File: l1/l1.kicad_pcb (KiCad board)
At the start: 2 copper layers, 122 x 122 mm, 60 parts

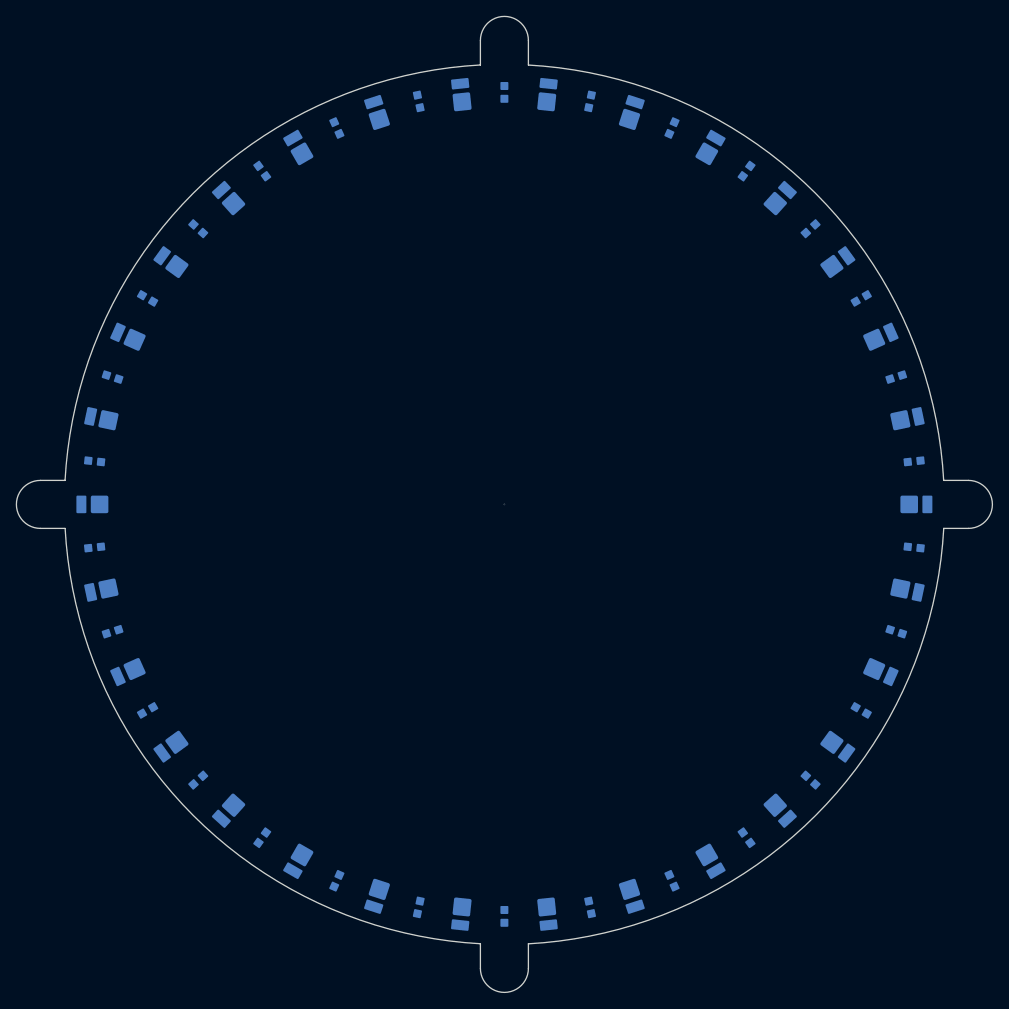
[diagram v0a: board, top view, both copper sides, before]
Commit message: 死
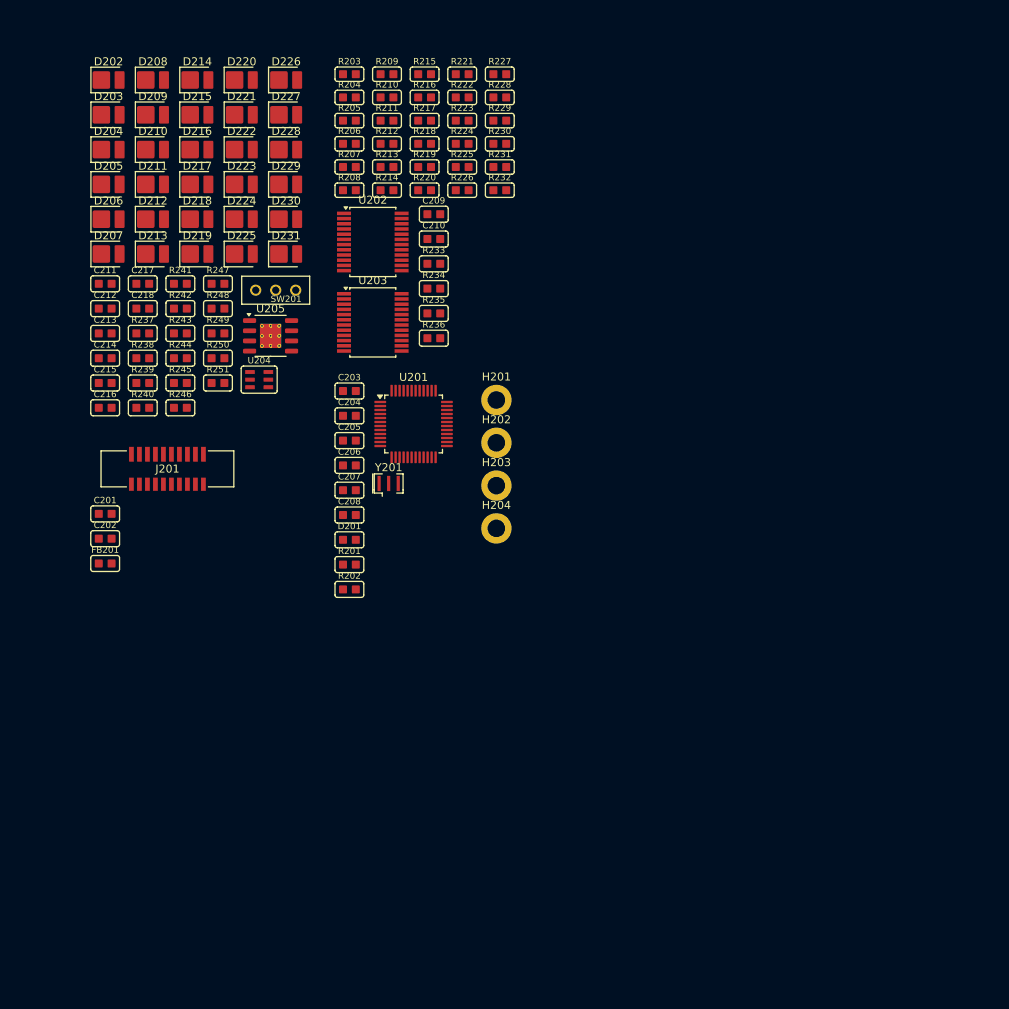
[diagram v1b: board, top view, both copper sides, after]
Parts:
- removed R252, R253, R254, R255, R256, R257, R258, R259, R260, R261, R262, R263, R264: R, Library:res0603
- added C201: 2u2, Library:cap0603, F.Cu at (105.3, 111.2)
- added C202: 2u2, Library:cap0603, F.Cu at (105.3, 114.3)
- added C203: 2u2, Library:cap0603, F.Cu at (135.8, 95.8)
- added C204: 0u1, Library:cap0603, F.Cu at (135.8, 98.9)
- added C205: 0u1, Library:cap0603, F.Cu at (135.8, 102.0)
- added C206: 0u1, Library:cap0603, F.Cu at (135.8, 105.1)
- added C207: 0u1, Library:cap0603, F.Cu at (135.8, 108.2)
- added C208: 0u1, Library:cap0603, F.Cu at (135.8, 111.3)
- added C209: 0u1, Library:cap0603, F.Cu at (146.4, 73.7)
- added C210: 0u1, Library:cap0603, F.Cu at (146.4, 76.8)
- added C211: 0u1, Library:cap0603, F.Cu at (105.3, 82.4)
- added C212: 10n, Library:cap0603, F.Cu at (105.3, 85.5)
- added C213: 10u, Library:cap0603, F.Cu at (105.3, 88.6)
- added C214: 22u, Library:cap0603, F.Cu at (105.3, 91.7)
- added C215: 0u1, Library:cap0603, F.Cu at (105.3, 94.8)
- added C216: 22u, Library:cap0603, F.Cu at (105.3, 97.9)
- added C217: 1u, Library:cap0603, F.Cu at (110.0, 82.4)
- added C218: 0u1, Library:cap0603, F.Cu at (110.0, 85.5)
- added D231: LED, Library:led2835, F.Cu at (127.9, 78.7)
- added FB201: 100R, Library:fb0603, F.Cu at (105.3, 117.4)
- added H201: MountingHole, MountingHole:MountingHole_2.2mm_M2_ISO14580_Pad, F.Cu at (154.2, 97.0)
- added H202: MountingHole, MountingHole:MountingHole_2.2mm_M2_ISO14580_Pad, F.Cu at (154.2, 102.3)
- added H203: MountingHole, MountingHole:MountingHole_2.2mm_M2_ISO14580_Pad, F.Cu at (154.2, 107.7)
- added H204: MountingHole, MountingHole:MountingHole_2.2mm_M2_ISO14580_Pad, F.Cu at (154.2, 113.0)
- added J201: Conn_01x10, Library:526101071, F.Cu at (113.1, 105.6)
- added R201: R, Library:res0603, F.Cu at (135.8, 117.5)
- added R202: 1K, Library:res0603, F.Cu at (135.8, 120.6)
- added R203: R_Photo, Library:als-pt19, F.Cu at (135.8, 56.2)
- added R204: R_Photo, Library:als-pt19, F.Cu at (135.8, 59.1)
- added R205: R_Photo, Library:als-pt19, F.Cu at (135.8, 62.0)
- added R206: R_Photo, Library:als-pt19, F.Cu at (135.8, 64.9)
- added R207: R_Photo, Library:als-pt19, F.Cu at (135.8, 67.8)
- added R208: R_Photo, Library:als-pt19, F.Cu at (135.8, 70.7)
- added R209: R_Photo, Library:als-pt19, F.Cu at (140.5, 56.2)
- added R210: R_Photo, Library:als-pt19, F.Cu at (140.5, 59.1)
- added R211: R_Photo, Library:als-pt19, F.Cu at (140.5, 62.0)
- added R212: R_Photo, Library:als-pt19, F.Cu at (140.5, 64.9)
- added R213: R_Photo, Library:als-pt19, F.Cu at (140.5, 67.8)
- added R214: R_Photo, Library:als-pt19, F.Cu at (140.5, 70.7)
- added R215: R_Photo, Library:als-pt19, F.Cu at (145.2, 56.2)
- added R216: R_Photo, Library:als-pt19, F.Cu at (145.2, 59.1)
- added R217: R_Photo, Library:als-pt19, F.Cu at (145.2, 62.0)
- added R218: R_Photo, Library:als-pt19, F.Cu at (145.2, 64.9)
- added R219: R_Photo, Library:als-pt19, F.Cu at (145.2, 67.8)
- added R220: R_Photo, Library:als-pt19, F.Cu at (145.2, 70.7)
- added R221: R_Photo, Library:als-pt19, F.Cu at (149.9, 56.2)
- added R222: R_Photo, Library:als-pt19, F.Cu at (149.9, 59.1)
- added R223: R_Photo, Library:als-pt19, F.Cu at (149.9, 62.0)
- added R224: R_Photo, Library:als-pt19, F.Cu at (149.9, 64.9)
- added R225: R_Photo, Library:als-pt19, F.Cu at (149.9, 67.8)
- added R226: R_Photo, Library:als-pt19, F.Cu at (149.9, 70.7)
- added R227: R_Photo, Library:als-pt19, F.Cu at (154.6, 56.2)
- added R228: R_Photo, Library:als-pt19, F.Cu at (154.6, 59.1)
- added R229: R_Photo, Library:als-pt19, F.Cu at (154.6, 62.0)
- added R230: R_Photo, Library:als-pt19, F.Cu at (154.6, 64.9)
- added R231: R_Photo, Library:als-pt19, F.Cu at (154.6, 67.8)
- added R232: R_Photo, Library:als-pt19, F.Cu at (154.6, 70.7)
- added R233: 3K24, Library:res0603, F.Cu at (146.4, 79.9)
- added R234: 10K, Library:res0603, F.Cu at (146.4, 83.0)
- added SW201: SW_SPDT, Library:SS12D00G3, F.Cu at (126.6, 83.2)
- added U201: STM32F103CBTX, Package_QFP:LQFP-48_7x7mm_P0.5mm, F.Cu at (143.8, 100.0)
- added U202: CD74HC4067SM, Package_SO:SSOP-24_5.3x8.2mm_P0.65mm, F.Cu at (138.8, 77.2)
- added U203: CD74HC4067SM, Package_SO:SSOP-24_5.3x8.2mm_P0.65mm, F.Cu at (138.8, 87.2)
- added U204: TPS22917x, Library:SOT-23-6, F.Cu at (124.5, 94.4)
- added U205: ILD8150, Package_SO:Infineon_PG-DSO-8-27_3.9x4.9mm_EP2.65x3mm_ThermalVias, F.Cu at (126.0, 88.9)
- added Y201: 8Mhz, Crystal:Resonator_SMD_Murata_CSTxExxV-3Pin_3.0x1.1mm, F.Cu at (140.7, 107.4)
- D201: value LED -> RED; footprint Library:led2835 -> Library:led0603; moved to F.Cu
- D202, D203, D204, D205, D206, D207, D208, D209, D210, D211, D212, D213, D214, D215, D216, D217, D218, D219, D220, D221, D222, D223, D224, D225, D226, D227, D228, D229, D230, R250: moved to F.Cu
- R235: value R -> 3K24; moved to F.Cu
- R236, R249: value R -> 10K; moved to F.Cu
- R237, R238, R239, R240, R241, R242, R243, R244, R245, R246: value R -> 150; moved to F.Cu
- R247: value R -> 100K; moved to F.Cu
- R248: value R -> 1; moved to F.Cu
- R251: value R -> 0.3; moved to F.Cu
- moved D214 113.0 mm to (116.8, 57.0), turned to 0 degrees
- moved D209 111.4 mm to (111.3, 61.3), turned to 0 degrees
- moved D208 111.2 mm to (111.3, 57.0), turned to 0 degrees
- moved D210 110.9 mm to (111.3, 65.7), turned to 0 degrees
- moved D211 109.6 mm to (111.3, 70.0), turned to 0 degrees
- moved D212 107.7 mm to (111.3, 74.3), turned to 0 degrees
- moved D215 106.8 mm to (116.8, 61.3), turned to 0 degrees
- moved D213 105.4 mm to (111.3, 78.7), turned to 0 degrees
- moved D216 100.2 mm to (116.8, 65.7)
- moved R241 99.5 mm to (114.7, 82.4), turned to 0 degrees
- moved R240 97.4 mm to (110.0, 97.9), turned to 0 degrees
- moved R239 97.1 mm to (110.0, 94.8), turned to 0 degrees
- moved R242 96.5 mm to (114.7, 85.5), turned to 0 degrees
- moved R238 96.4 mm to (110.0, 91.7), turned to 0 degrees
- moved R237 95.2 mm to (110.0, 88.6), turned to 0 degrees
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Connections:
- D201 pad 2: +3V3 -> /Light Ring/STM32/MCU1 LED
- D202 pad 1: Net-(D201-K) -> Net-(D202-K)
- D202 pad 2: +3V3 -> /Light Ring/LED/LED VIN
- D203 pad 1: Net-(D201-K) -> Net-(D203-K)
- D203 pad 2: +3V3 -> /Light Ring/LED/LED VIN
- D204 pad 1: Net-(D201-K) -> Net-(D204-K)
- D204 pad 2: +3V3 -> /Light Ring/LED/LED VIN
- D205 pad 1: Net-(D201-K) -> Net-(D205-K)
- D205 pad 2: +3V3 -> /Light Ring/LED/LED VIN
- D206 pad 1: Net-(D201-K) -> Net-(D206-K)
- D206 pad 2: +3V3 -> /Light Ring/LED/LED VIN
- D207 pad 1: Net-(D201-K) -> Net-(D207-K)
- D207 pad 2: +3V3 -> /Light Ring/LED/LED VIN
- D208 pad 1: Net-(D201-K) -> Net-(D208-K)
- D208 pad 2: +3V3 -> /Light Ring/LED/LED VIN
- D209 pad 1: Net-(D201-K) -> Net-(D209-K)
- D209 pad 2: +3V3 -> /Light Ring/LED/LED VIN
- D210 pad 1: Net-(D201-K) -> Net-(D210-K)
- D210 pad 2: +3V3 -> /Light Ring/LED/LED VIN
- D211 pad 1: Net-(D201-K) -> Net-(D211-K)
- D211 pad 2: +3V3 -> /Light Ring/LED/LED VIN
- D212 pad 1: Net-(D201-K) -> Net-(D212-K)
- D212 pad 2: +3V3 -> Net-(D202-K)
- D213 pad 1: Net-(D201-K) -> Net-(D213-K)
- D213 pad 2: +3V3 -> Net-(D203-K)
- D214 pad 1: Net-(D201-K) -> Net-(D214-K)
- D214 pad 2: +3V3 -> Net-(D204-K)
- D215 pad 1: Net-(D201-K) -> Net-(D215-K)
- D215 pad 2: +3V3 -> Net-(D205-K)
- D216 pad 1: Net-(D201-K) -> Net-(D216-K)
- D216 pad 2: +3V3 -> Net-(D206-K)
- D217 pad 1: Net-(D201-K) -> Net-(D217-K)
- D217 pad 2: +3V3 -> Net-(D207-K)
- D218 pad 1: Net-(D201-K) -> Net-(D218-K)
- D218 pad 2: +3V3 -> Net-(D208-K)
- D219 pad 1: Net-(D201-K) -> Net-(D219-K)
- D219 pad 2: +3V3 -> Net-(D209-K)
- D220 pad 1: Net-(D201-K) -> Net-(D220-K)
- D220 pad 2: +3V3 -> Net-(D210-K)
- D221 pad 1: Net-(D201-K) -> Net-(D221-K)
- D221 pad 2: +3V3 -> Net-(D211-K)
- D222 pad 1: Net-(D201-K) -> Net-(D222-K)
- D222 pad 2: +3V3 -> Net-(D212-K)
- D223 pad 1: Net-(D201-K) -> Net-(D223-K)
- D223 pad 2: +3V3 -> Net-(D213-K)
- D224 pad 1: Net-(D201-K) -> Net-(D224-K)
- D224 pad 2: +3V3 -> Net-(D214-K)
- D225 pad 1: Net-(D201-K) -> Net-(D225-K)
- D225 pad 2: +3V3 -> Net-(D215-K)
- D226 pad 1: Net-(D201-K) -> Net-(D226-K)
- D226 pad 2: +3V3 -> Net-(D216-K)
- D227 pad 1: Net-(D201-K) -> Net-(D227-K)
- D227 pad 2: +3V3 -> Net-(D217-K)
- D228 pad 1: Net-(D201-K) -> Net-(D228-K)
- D228 pad 2: +3V3 -> Net-(D218-K)
- D229 pad 1: Net-(D201-K) -> Net-(D229-K)
- D229 pad 2: +3V3 -> Net-(D219-K)
- D230 pad 1: Net-(D201-K) -> Net-(D230-K)
- D230 pad 2: +3V3 -> Net-(D220-K)
- R235 pad 1: Net-(D201-K) -> GNDREF
- R235 pad 2: GNDREF -> /Light Ring/MUX/M2
- R236 pad 1: Net-(D201-K) -> GNDREF
- R236 pad 2: GNDREF -> Net-(U203-~{E})
- R237 pad 1: Net-(D201-K) -> Net-(D222-K)
- R237 pad 2: GNDREF -> /Light Ring/LED/LED VOUT
- R238 pad 1: Net-(D201-K) -> Net-(D223-K)
- R238 pad 2: GNDREF -> /Light Ring/LED/LED VOUT
- R239 pad 1: Net-(D201-K) -> Net-(D224-K)
- R239 pad 2: GNDREF -> /Light Ring/LED/LED VOUT
- R240 pad 1: Net-(D201-K) -> Net-(D225-K)
- R240 pad 2: GNDREF -> /Light Ring/LED/LED VOUT
- R241 pad 1: Net-(D201-K) -> Net-(D226-K)
- R241 pad 2: GNDREF -> /Light Ring/LED/LED VOUT
- R242 pad 1: Net-(D201-K) -> Net-(D227-K)
- R242 pad 2: GNDREF -> /Light Ring/LED/LED VOUT
- R243 pad 1: Net-(D201-K) -> Net-(D228-K)
- R243 pad 2: GNDREF -> /Light Ring/LED/LED VOUT
- R244 pad 1: Net-(D201-K) -> Net-(D229-K)
- R244 pad 2: GNDREF -> /Light Ring/LED/LED VOUT
- R245 pad 1: Net-(D201-K) -> Net-(D230-K)
- R245 pad 2: GNDREF -> /Light Ring/LED/LED VOUT
- R246 pad 1: Net-(D201-K) -> Net-(D231-K)
- R246 pad 2: GNDREF -> /Light Ring/LED/LED VOUT
- R247 pad 1: Net-(D201-K) -> Net-(U204-VOUT)
- R247 pad 2: GNDREF -> Net-(U204-QOD)
- R248 pad 1: Net-(D201-K) -> /Light Ring/LED/LED VOUT
- R248 pad 2: GNDREF -> Net-(R248-Pad2)
- R249 pad 1: Net-(D201-K) -> +3V3 FLIT
- R249 pad 2: GNDREF -> Net-(SW201-B)
- R250 pad 1: Net-(D201-K) -> Net-(SW201-B)
- R250 pad 2: GNDREF -> /Light Ring/LED/LED PWR
- R251 pad 1: Net-(D201-K) -> Net-(R248-Pad2)
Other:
- board outline removed
- rule pad_to_mask_clearance: 0 -> 0.15
